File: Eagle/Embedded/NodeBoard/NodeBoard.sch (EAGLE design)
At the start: 68 parts, among them IC1 7812TV, IC2 5v, IC3 3v3, IC4 REG1117, IC5 REG1117, J1 DCJ0202, Q2 IRF740, T1 BC547

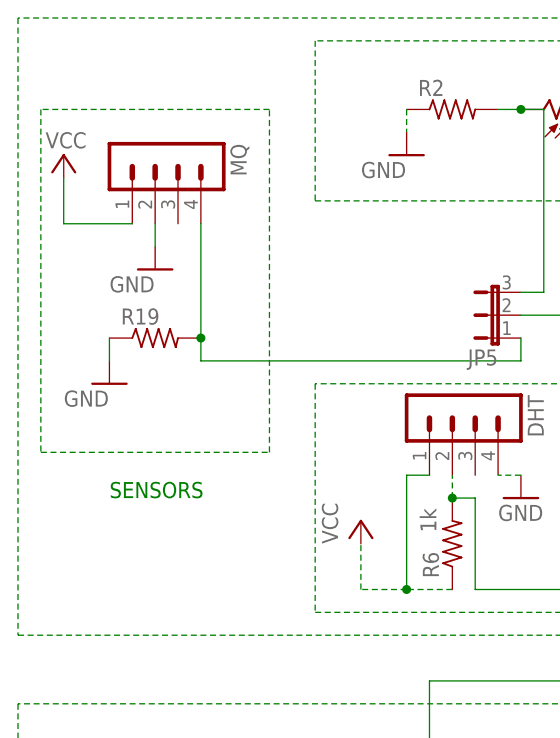
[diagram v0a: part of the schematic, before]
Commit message: Minor Eagle Board fixes
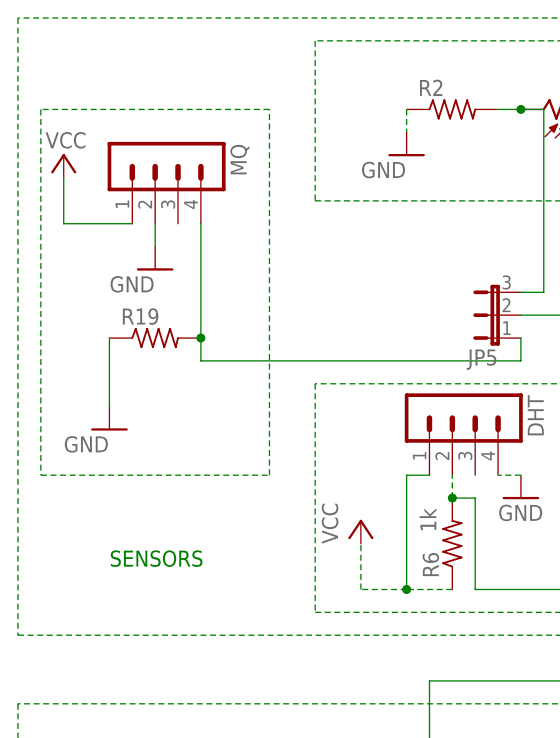
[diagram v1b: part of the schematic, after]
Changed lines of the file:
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@@
 <text x="139.7" y="-76.2" size="1.778" layer="91">220V AC IN</text>
 <text x="320.04" y="83.82" size="1.778" layer="91">CONTROLS AND PROGRAMMING</text>
-<text x="114.3" y="43.18" size="1.778" layer="91">SENSORS</text>
+<text x="114.3" y="35.56" size="1.778" layer="91">SENSORS</text>
 <text x="358.14" y="-73.66" size="3.81" layer="91">1.0</text>
 <text x="269.24" y="-50.8" size="2.54" layer="91">Embedded system based on ESP8266 12E microcontroller</text>
@@
 <instance part="JP5" gate="1" x="157.48" y="63.5" rot="R90"/>
 <instance part="R19" gate="G$1" x="119.38" y="60.96"/>
-<instance part="GND6" gate="1" x="114.3" y="55.88" smashed="yes">
-<attribute name="VALUE" x="109.22" y="53.34" size="1.778" layer="96"/>
+<instance part="GND6" gate="1" x="114.3" y="50.8" smashed="yes">
+<attribute name="VALUE" x="109.22" y="48.26" size="1.778" layer="96"/>
 </instance>
 <instance part="GND21" gate="1" x="345.44" y="-12.7"/>
@@
 <pinref part="GND6" gate="1" pin="GND"/>
 <pinref part="R19" gate="G$1" pin="1"/>
-<wire x1="114.3" y1="58.42" x2="114.3" y2="60.96" width="0.1524" layer="91"/>
+<wire x1="114.3" y1="53.34" x2="114.3" y2="60.96" width="0.1524" layer="91"/>
 </segment>
 <segment>
@@
 <net name="N$23" class="0">
 <segment>
-<wire x1="106.68" y1="86.36" x2="106.68" y2="48.26" width="0.1524" layer="91" style="shortdash"/>
-<wire x1="106.68" y1="48.26" x2="132.08" y2="48.26" width="0.1524" layer="91" style="shortdash"/>
-<wire x1="132.08" y1="48.26" x2="132.08" y2="86.36" width="0.1524" layer="91" style="shortdash"/>
+<wire x1="106.68" y1="86.36" x2="106.68" y2="45.72" width="0.1524" layer="91" style="shortdash"/>
+<wire x1="106.68" y1="45.72" x2="132.08" y2="45.72" width="0.1524" layer="91" style="shortdash"/>
+<wire x1="132.08" y1="45.72" x2="132.08" y2="86.36" width="0.1524" layer="91" style="shortdash"/>
 <wire x1="132.08" y1="86.36" x2="106.68" y2="86.36" width="0.1524" layer="91" style="shortdash"/>
 </segment>

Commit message: Report, and eagle changes
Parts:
- removed C4: 0u33, resistor:CPOL-USE2,5-6E
- removed IC2: 5v, v-reg:LM317TS
- removed IC3: 3v3, v-reg:LM317TS
- removed JMP4: 0R-JUMPA, jump-0r-smd:0R-JUMPA
- removed JP1: (no value), jumper:JP1E
- removed LED3: (no value), adafruit:LEDCHIPLED_1206
- removed LED5: RED, led:LED5MM
- removed MODE_SEL: (no value), special:SW_DIP-4
- removed PLD: VT23N2, photo-elements:VT23N2
- removed R11: 160, resistor:R-EU_R0603
- removed R13: 160, rcl:R-US_0204/7
- removed R3, R4, R5: 10k, rcl:R-US_0204/7
- added D5, D6: 1N4004, adafruit:1N4004
- added JP10, JP8, JP9: (no value), jumper:JP4E
- added LM317: 3v3, v-reg:LM317TS
- added LM317T: 5v, v-reg:LM317TS
- added Q1, Q3: IRF740, transistor-power:IRF740
- added R21: 1k, rcl:R-US_0204/7
- added SD_CARD: (no value), con-lstb:MA06-1
- added T2: BC547, transistor:BC547
- added U$4: RELAY, relay:RELAY
- added X3, X5, X6: (no value), con-wago-500:W237-103
- added X4: (no value), con-wago-500:W237-102
- JP2: device jumper:JP2E -> jumper:JP4E
- JP5: device jumper:JP2E -> jumper:JP1E
- R1: device rcl:R-US_0204/7 -> resistor:R-EU_R0603
- R2: value (none) -> 10k; device rcl:R-US_0204/7 -> resistor:R-EU_R0603
- U$1: device RELAY:RELAY -> relay:RELAY
- X1: device con-wago-500:W237-6 -> con-wago-500:W237-102
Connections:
- net N$12 renamed TX
- net N$13 renamed RX
- net N$15 renamed GPIO12
- removed net N$14: MODE_SEL.6, R5.2, U1.GPIO4
- removed net N$16: MODE_SEL.8, R4.2, U1.GPIO15
- removed net N$21: JP1.1, U1.GPIO16
- removed net N$25: JP5.3, PLD.1, R2.2
- removed net N$26: U$1.COM, X1-1.KL
- removed net N$27: JP2.2, U1.GPIO14
- removed net N$29: JP1.2, R8.1, U$5.2, U1.RESET
- removed net N$3: JP5.2, U1.ADC
- removed net N$32: LED3.A, R11.2
- removed net N$34: LED5.A, R13.1
- removed net N$35: JMP3-0R.2, U1.*GPIO10
- removed net N$38: JMP4-0R.2, U1.GPIO13
- removed net N$39: JMP4-0R.3, R11.1
- removed net N$40: JMP4-0R.1, R13.2
- removed net N$59: JP2.1, Q2.G
- removed net N$6: U$1.COM-OPEN, U$2.PRI_2, U$3.P$2
- removed net N$7: X1-3.KL, X1-4.KL
- new net 12V_IN: D6.A, J1.1, X1-2.KL, X2-2.KL, X4-2.KL
- new net AC_C: U$2.PRI_1, X3-2.KL, X6-1.KL, X6-2.KL
- new net AC_G: X3-1.KL, X5-1.KL, X6-3.KL
- new net AC_P: U$1.COM-OPEN, U$2.PRI_2, U$3.P$2, U$4.COM-OPEN
- new net ADC: MQ.4, R19.2, U1.ADC
- new net CS: SD_CARD.5, U1.CS0
- new net GPIO0: Q2.G, R9.1, U$6.1, U1.GPIO0
- new net GPIO10: JP9.4, U1.*GPIO10
- new net GPIO13: JP10.4, U1.GPIO13
- new net GPIO14: JP8.4, U1.GPIO14
- new net GPIO15: Q1.G, R1.2, U1.GPIO15
- new net GPIO16: JP2.4, U1.GPIO16
- new net GPIO2: Q3.G, R2.2, U1.GPIO2
- new net GPIO4: R21.2, U1.GPIO4
- new net GPIO5: R14.2, U1.GPIO5
- new net GPIO9: JMP3-0R.2, U1.*GPIO9
- new net MISO: SD_CARD.2, U1.MISO
- new net MOSI: SD_CARD.4, U1.MOSI
- new net RST: R8.1, U$5.2, U1.RESET
- new net SCLK: SD_CARD.3, U1.SCLK
- net 12V: now also D6.C; no longer J1.1, X2-2.KL
- net 19V: no longer C4.+
- net 3V3: now also JP10.2, JP2.2, JP8.2, JP9.2, MQ.1, R2.1, SD_CARD.6; no longer MODE_SEL.1, MODE_SEL.2, MODE_SEL.3, MODE_SEL.4
- net GND: now also JP10.3, JP2.3, JP8.3, JP9.3, Q1.S, Q3.S, SD_CARD.1, T2.E; no longer C4.-, LED3.C, LED5.C, R2.1, R3.1, R4.1, R5.1
- net N$18: now also Q1.D, X1-1.KL; no longer MODE_SEL.5, R3.2, U1.GPIO5
- net N$22: now also Q3.D, X4-1.KL; no longer U$6.2, U1.GPIO0
- net N$44: now also R21.1, T2.B; no longer JP2.3, R14.2
- net N$45: now also LM317T.OUT; no longer IC2.OUT
- net N$46: now also LM317T.ADJ; no longer IC2.ADJ
- net N$47: now also LM317.OUT; no longer IC3.OUT
- net N$48: now also LM317.ADJ; no longer IC3.ADJ
- net N$49: now also LM317T.IN; no longer IC2.IN
- net N$50: now also LM317.IN; no longer IC3.IN
- net N$60: now also D5.A, T2.C, U$4.GND; no longer MODE_SEL.7, R1.2, U1.GPIO2
- net N$62: now also X3-3.KL; no longer X1-6.KL
- net N$63: now also U$4.COM, X5-2.KL; no longer R9.1, U$6.1
- net N$8: now also U$1.COM, X5-3.KL; no longer U$2.PRI_1, X1-2.KL, X1-5.KL
- net N$9: now also JP5.2, MQ.3; no longer JP5.1, MQ.4, R19.2
- net VCC: now also D5.C, JP10.1, JP2.1, JP5.1, JP8.1, JP9.1, U$4.IN; no longer MQ.1, PLD.2
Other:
- note added: "3.0"
- note added: "BLACK-BOX COMPONENTS"
- note added: "EXTRA IN/OUT PINS"
- note added: "MAIN BRAIN"
- note added: "Mesh-Network (Node/Base Station)"
- note added: "SD CARD READER (ONLY FOR END NODE)"
- note added: "STANDARD INPUTS"
- note added: "STANDARD OUTPUTS"
- note removed: "1.0"
- moved on the sheet: B1, C1, C2, C3, C5, C6, C7, C8, C9, D1, D2, D3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
